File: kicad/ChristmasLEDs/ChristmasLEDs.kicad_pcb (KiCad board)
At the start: 2 copper layers, 42.4 x 66.6 mm, 21 parts, among them J1 Power In, J2 PIR Motion In, J3 AC Relay Out, J4 WS2812 LED Out, J6 Button In, U1 74HC245

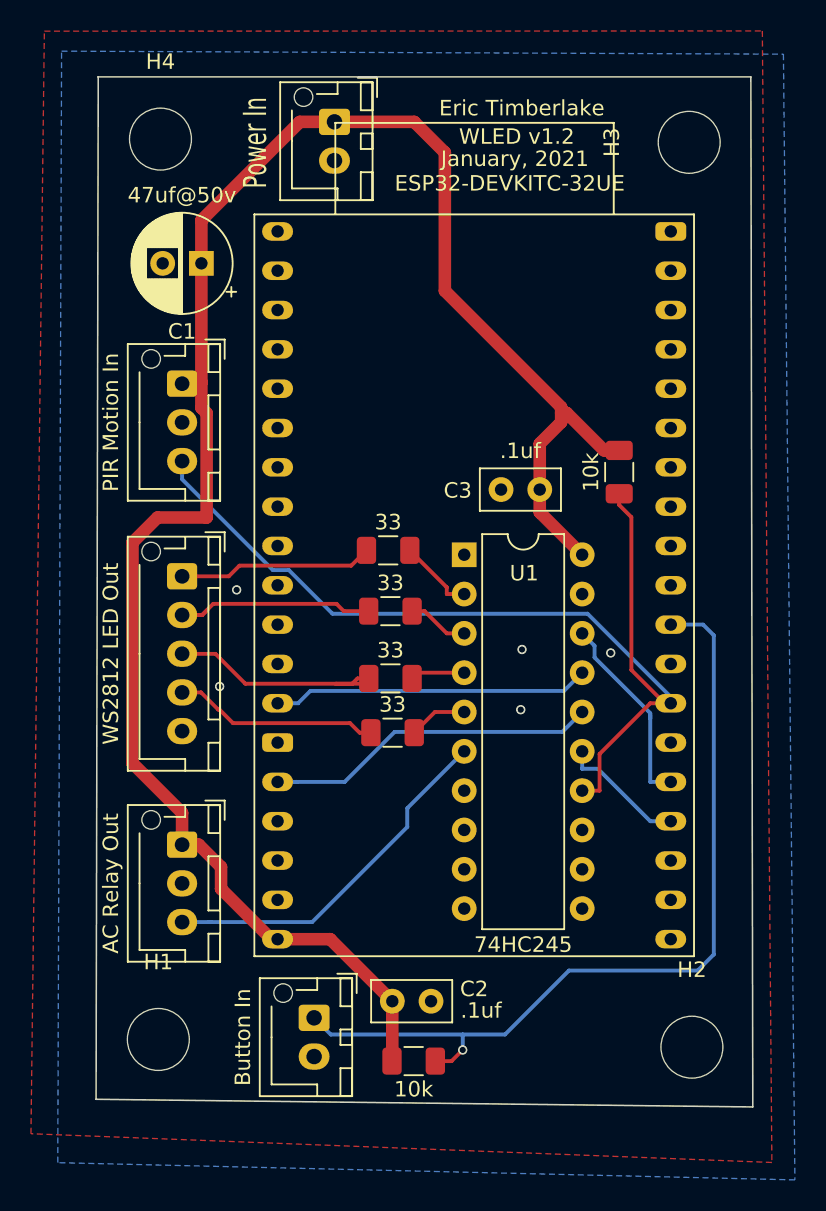
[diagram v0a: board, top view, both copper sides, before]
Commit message: Update board error!!
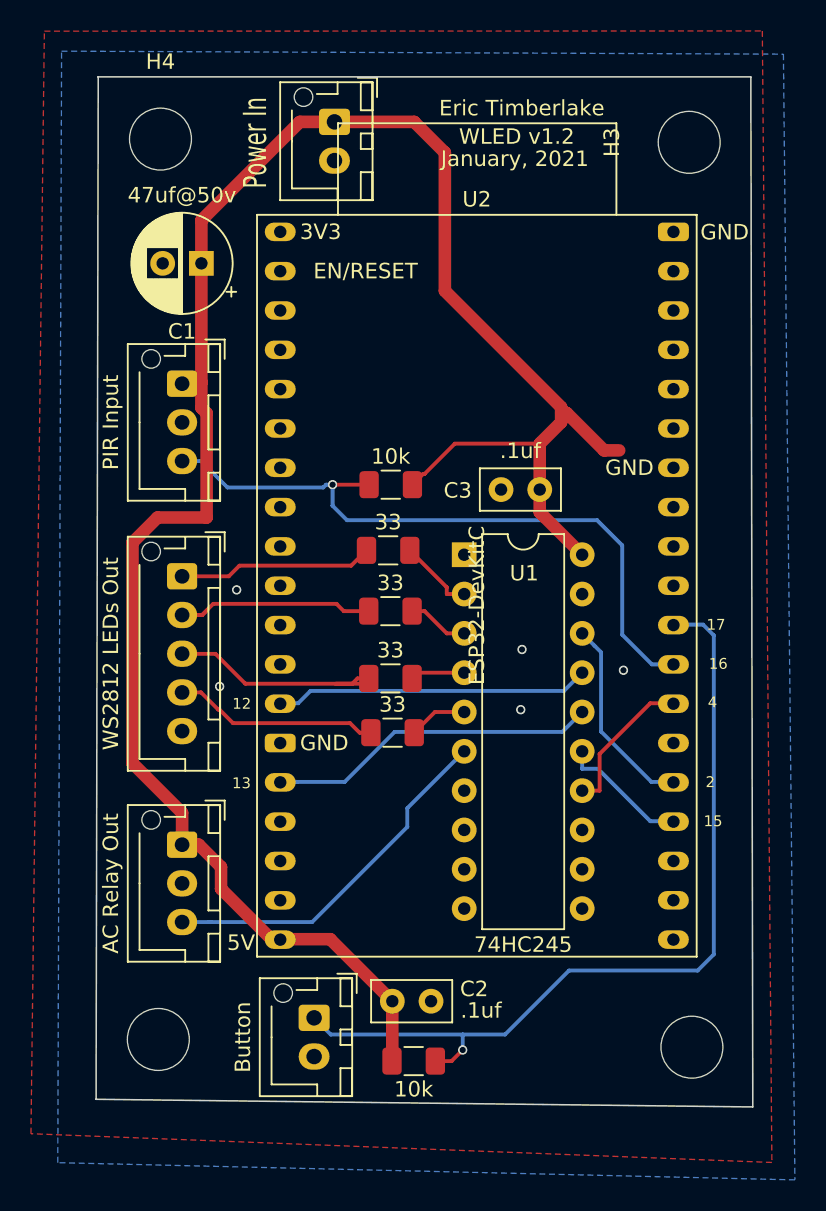
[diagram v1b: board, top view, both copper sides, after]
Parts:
- removed ESP32-DEVKITC-32UE: ESP32-DevKitC, Espressif:ESP32-DevKitC
- added U2: ESP32-DevKitC, Espressif:ESP32-DevKitC, F.Cu at (155.9, 69.4)
- J2: value PIR Motion In -> PIR Input
- J4: value WS2812 LED Out -> WS2812 LEDs Out
- J6: value Button In -> Button
- moved R5 14.8 mm to (163.0, 85.7), turned to 180 degrees
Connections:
- J2 pad 3: /GPIO4 -> /GPIO16
- R5 pad 2: /GPIO4 -> /GPIO16
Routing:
- net /GPIO4: track 63.6 -> 9.85 mm
- net /GPIO16: track 0.00 -> 43.9 mm, vias 0 -> 1
- net +5V: track 145.2 -> 154.6 mm
